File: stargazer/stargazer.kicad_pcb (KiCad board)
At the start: 2 copper layers, 72 x 40.8 mm, 81 parts, among them J1 1935161, J2 10118193-0001LF, J3 Conn_01x02_Pin, J4 1935161, J5 CON-SMA-EDGE-S, J6 MSD-1-A, SW1 JS202011SCQN, U1 ESP32-C3-WROOM-02, U10 LPS22DF, U11 KX134, U12 LIS3MDL, U13 LSM6DSO, U2 MCP73831-2-OT, U3 USBLC6-2SC6, U4 LM66100DCKR, U5 LM66100DCKR, U6 AP2112K-3.3, U7 W25Q128JVSIQ, U8 SAM-M10Q, U9 RFM95W-868S2

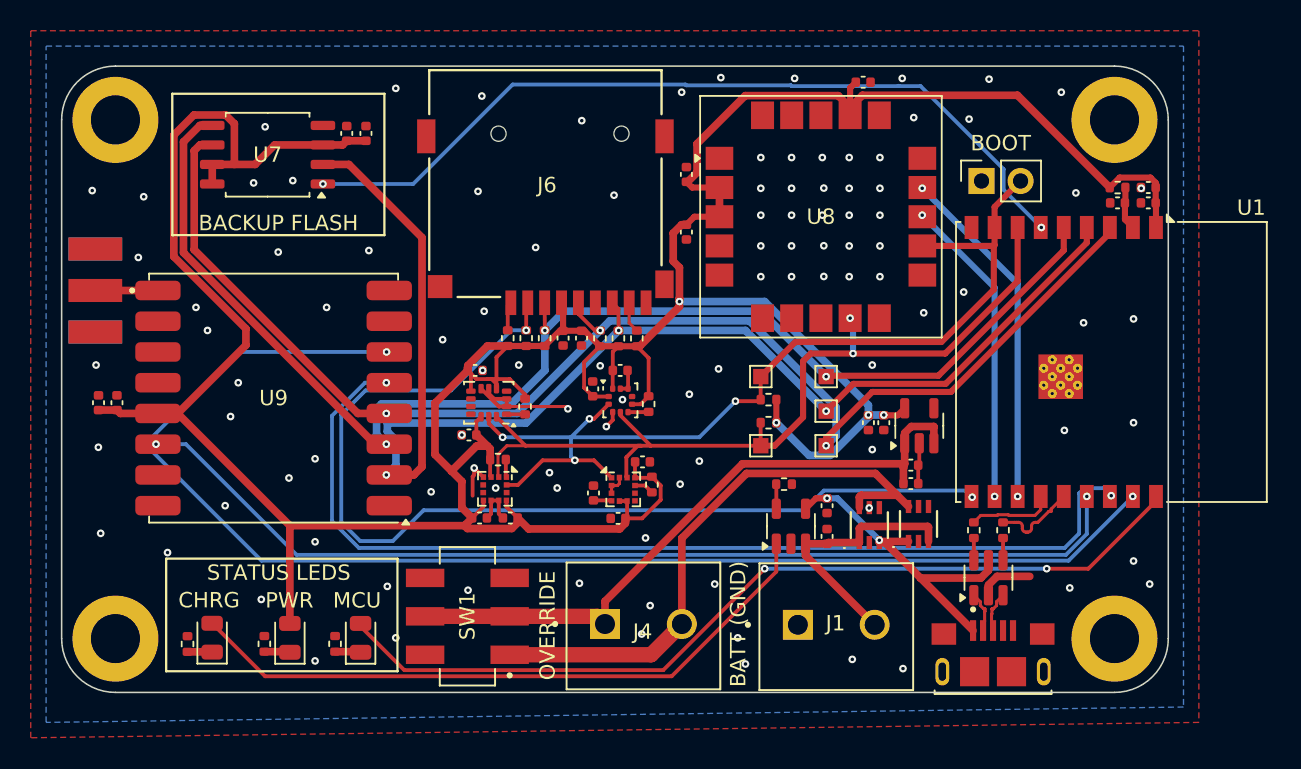
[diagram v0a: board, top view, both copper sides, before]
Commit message: Revision B
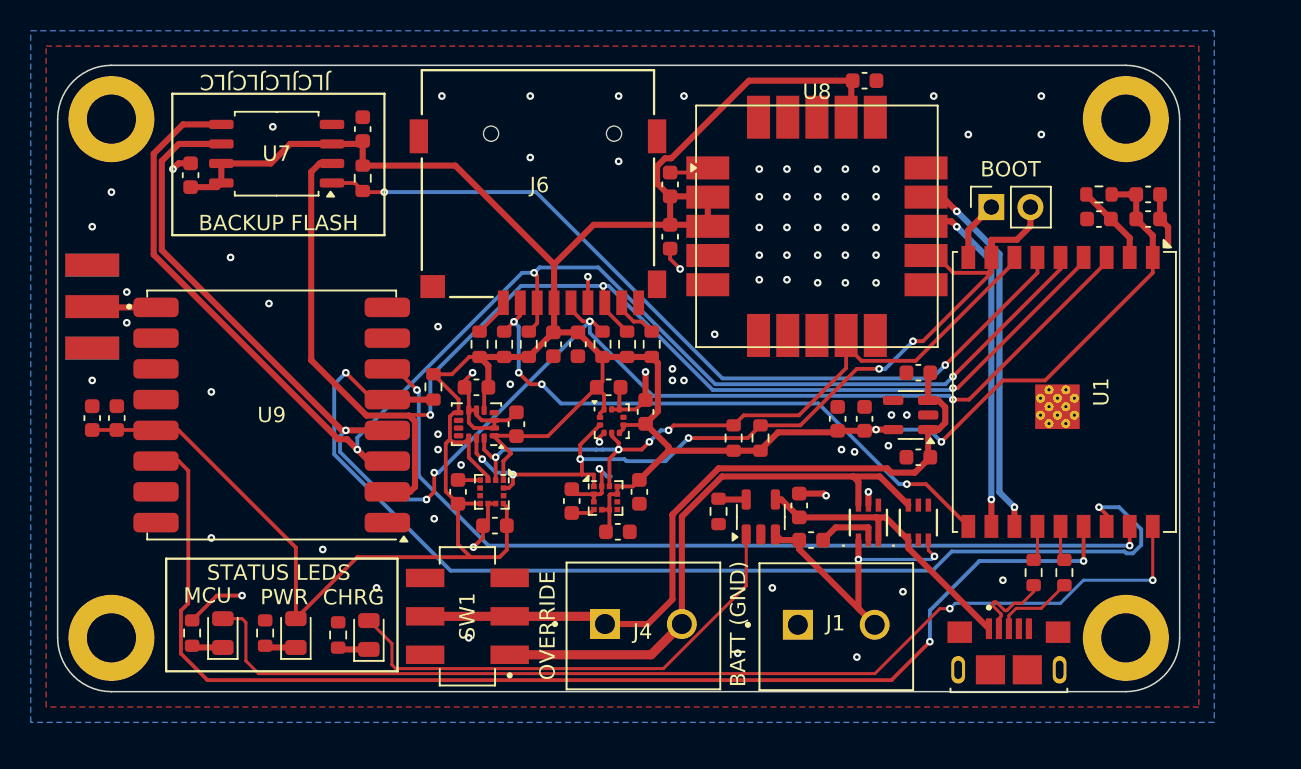
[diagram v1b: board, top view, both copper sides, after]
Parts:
- removed D4: SML-LX1206SRC-TR, LED_SMD:LED_0805_2012Metric
- removed R18, R19: 0, Resistor_SMD:R_0402_1005Metric
- removed TP1: SPI CLK, TestPoint:TestPoint_Pad_1.0x1.0mm
- removed TP2: SPI MOSI, TestPoint:TestPoint_Pad_1.0x1.0mm
- removed TP3: SPI MISO, TestPoint:TestPoint_Pad_1.0x1.0mm
- removed TP4: I2C SDA, TestPoint:TestPoint_Pad_1.0x1.0mm
- removed TP5: I2C SCL, TestPoint:TestPoint_Pad_1.0x1.0mm
- removed U3: USBLC6-2SC6, Package_TO_SOT_SMD:SOT-23-6
- added D3: SML-LX1206SRC-TR, LED_SMD:LED_0805_2012Metric, F.Cu at (119.5, 111.2)
- C1, C10, C11, C12, C13, C14, C15, C16, C17, C18, C19, C2, C20, C21, C22, C23, C24, C25, C26, C27, C3, C4, C5, C6, C7, C8, C9: footprint Capacitor_SMD:C_0402_1005Metric -> Capacitor_SMD:C_0603_1608Metric
- R1, R11, R12, R13, R14, R15, R16, R2, R3, R4, R5, R6, R7, R8: footprint Resistor_SMD:R_0402_1005Metric -> Resistor_SMD:R_0603_1608Metric
- R10: value 470 -> 4k7; footprint Resistor_SMD:R_0402_1005Metric -> Resistor_SMD:R_0603_1608Metric
- R17: value 0 -> 4k7; footprint Resistor_SMD:R_0402_1005Metric -> Resistor_SMD:R_0603_1608Metric
- R9: value 0 -> 470; footprint Resistor_SMD:R_0402_1005Metric -> Resistor_SMD:R_0603_1608Metric
- U1: value ESP32-C3-WROOM-02 -> ESP32-C3-WROOM-02U-N4; footprint RF_Module:ESP32-C3-WROOM-02 -> RF_Module:ESP32-C3-WROOM-02U
- U8: footprint RF_GPS:ublox_SAM-M8Q -> 1935161:ublox_SAM-M10Q
- moved R10 30.3 mm to (128.6, 81.6), turned to -90 degrees
- moved R9 22.9 mm to (117.5, 111.2), turned to 90 degrees
- moved R17 14.5 mm to (136.2, 92.4)
- moved R11 13.6 mm to (133.2, 95.2)
- moved C14 11.7 mm to (117.4, 81.4)
- moved D2 10.2 mm to (129.0, 111.3)
- moved R8 9.82 mm to (127.0, 111.3)
- moved C6 6.03 mm to (164.8, 94.2), turned to 180 degrees
- moved R3 4.85 mm to (174.2, 107.2), turned to 90 degrees
- moved R4 4.77 mm to (172.2, 107.2), turned to 90 degrees
- moved R1 4.61 mm to (151.8, 103.3), turned to -90 degrees
- moved C26 4.41 mm to (138.6, 97.6), turned to 90 degrees
- moved R14 3.79 mm to (144.2, 92.4)
- moved C18 3.16 mm to (147.0, 96.8), turned to 90 degrees
- moved C24 3.14 mm to (136.0, 95.2)
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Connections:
- R10 pad 1: Net-(D4-K) -> +3V3
- R10 pad 2: GND -> CS_FLASH
- R11 pad 1: Net-(J6-DAT1) -> +3V3
- R11 pad 2: +3V3 -> CS_LORA
- R12 pad 1: MISO -> Net-(J6-DAT1)
- R13 pad 1: SCK -> MISO
- R14 pad 1: MOSI -> SCK
- R15 pad 1: CS_SD -> MOSI
- R16 pad 1: Net-(J6-DAT2) -> CS_SD
- R17 pad 1: +3V3 -> Net-(J6-DAT2)
- R17 pad 2: Net-(U12-SDO/SA1) -> +3V3
- R3 pad 1: JTAG_USB_P -> /Power Mangement And MCU/USB_P
- R3 pad 2: Net-(R3-Pad2) -> JTAG_USB_P
- R4 pad 1: JTAG_USB_N -> /Power Mangement And MCU/USB_N
- R4 pad 2: Net-(R4-Pad2) -> JTAG_USB_N
- R9 pad 1: +3V3 -> Net-(D3-K)
- R9 pad 2: Net-(U11-SDO/ADDR) -> GND
- U10 pad 5: Net-(U10-SA0) -> +3V3
- U11 pad 1: Net-(U11-SDO/ADDR) -> +3V3
- U12 pad 9: Net-(U12-SDO/SA1) -> +3V3
- U13 pad 1: Net-(U13-SDO/SA0) -> +3V3
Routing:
- net LORA_RST: track 87.4 -> 57.5 mm
- net GND: track 24.5 -> 51.9 mm, vias 106 -> 79
- net CS_SD: track 66.3 -> 39.1 mm, vias 2 -> 4
- net INT_LORA: track 66.6 -> 80.5 mm
- net +3V3: track 242.3 -> 230.2 mm, vias 4 -> 2
- net LED_STATUS: track 58.0 -> 69.5 mm
- net BATT_STAT: track 42.8 -> 32.2 mm
- net SDA: track 57.8 -> 48.7 mm, vias 2 -> 4
- net SCK: track 89.0 -> 97.6 mm, vias 3 -> 5
- net CS_LORA: track 66.2 -> 74.3 mm
- net MOSI: track 87.8 -> 94.8 mm
- net VDC: track 43.0 -> 48.3 mm
- net JTAG_USB_N: track 5.59 -> 2.28 mm
- net JTAG_USB_P: track 5.55 -> 2.28 mm
- net /Power Mangement And MCU/USB_N: track 2.70 -> 5.80 mm
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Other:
- board size 72 x 40.8 mm -> 73 x 40.8 mm
- board text added: "Nick Coombe (www.quizque.ca) Rev. B"
- board text removed: "Nick Coombe (www.quizque.ca) Rev. A"

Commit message: Stargazer PCB print update
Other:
- board text removed: "PCB3D_BR_main"
- board text removed: "PCB3D_TL_main"
